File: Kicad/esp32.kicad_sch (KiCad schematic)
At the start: 25 parts, among them J2 Display, J3 LED, J7 UART, U11 ESP32-WROOM-32UE-N16, U16 XL1509-3.3

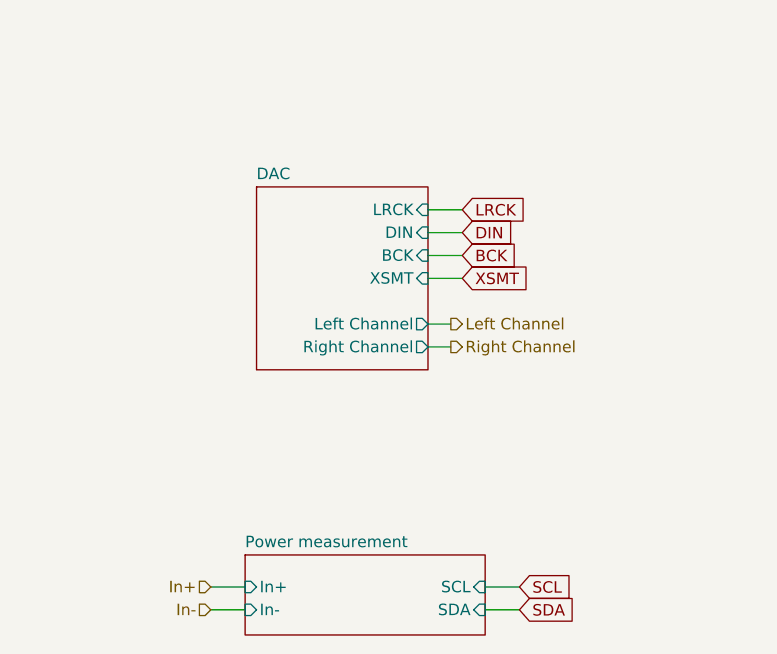
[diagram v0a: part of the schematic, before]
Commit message: final schematic
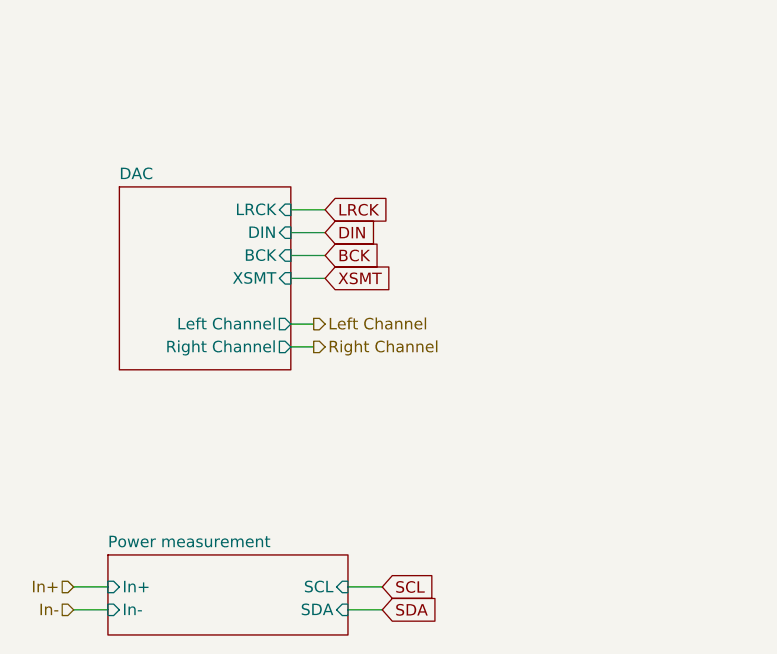
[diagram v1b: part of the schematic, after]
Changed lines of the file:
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@@
 	(wire
 		(pts
-			(xy 82.55 129.54) (xy 85.09 129.54)
+			(xy 67.31 129.54) (xy 69.85 129.54)
 		)
 		(stroke
@@
 	(wire
 		(pts
-			(xy 82.55 121.92) (xy 86.36 121.92)
+			(xy 67.31 121.92) (xy 71.12 121.92)
 		)
 		(stroke
@@
 	(wire
 		(pts
-			(xy 82.55 127) (xy 85.09 127)
+			(xy 67.31 127) (xy 69.85 127)
 		)
 		(stroke
@@
 	(wire
 		(pts
-			(xy 58.42 156.21) (xy 62.23 156.21)
+			(xy 43.18 156.21) (xy 46.99 156.21)
 		)
 		(stroke
@@
 	(wire
 		(pts
-			(xy 92.71 158.75) (xy 88.9 158.75)
+			(xy 77.47 158.75) (xy 73.66 158.75)
 		)
 		(stroke
@@
 	(wire
 		(pts
-			(xy 82.55 116.84) (xy 86.36 116.84)
+			(xy 67.31 116.84) (xy 71.12 116.84)
 		)
 		(stroke
@@
 	(wire
 		(pts
-			(xy 58.42 158.75) (xy 62.23 158.75)
+			(xy 43.18 158.75) (xy 46.99 158.75)
 		)
 		(stroke
@@
 	(wire
 		(pts
-			(xy 82.55 114.3) (xy 86.36 114.3)
+			(xy 67.31 114.3) (xy 71.12 114.3)
 		)
 		(stroke
@@
 	(wire
 		(pts
-			(xy 92.71 156.21) (xy 88.9 156.21)
+			(xy 77.47 156.21) (xy 73.66 156.21)
 		)
 		(stroke
@@
 	(wire
 		(pts
-			(xy 82.55 119.38) (xy 86.36 119.38)
+			(xy 67.31 119.38) (xy 71.12 119.38)
 		)
 		(stroke
@@
 	(global_label "BCK"
 		(shape input)
-		(at 86.36 119.38 0)
+		(at 71.12 119.38 0)
 		(fields_autoplaced yes)
 		(effects
@@
 		)
 		(property "Intersheetrefs" "${INTERSHEET_REFS}"
-			(at 93.1552 119.38 0)
+			(at 77.9152 119.38 0)
 			(hide yes)
 			(show_name no)
@@
 	(global_label "SCL"
 		(shape input)
-		(at 92.71 156.21 0)
+		(at 77.47 156.21 0)
 		(fields_autoplaced yes)
 		(effects
@@
 		)
 		(property "Intersheetrefs" "${INTERSHEET_REFS}"
-			(at 99.2028 156.21 0)
+			(at 83.9628 156.21 0)
 			(hide yes)
 			(show_name no)
@@
 	(global_label "XSMT"
 		(shape input)
-		(at 86.36 121.92 0)
+		(at 71.12 121.92 0)
 		(fields_autoplaced yes)
 		(effects
@@
 		)
 		(property "Intersheetrefs" "${INTERSHEET_REFS}"
-			(at 94.1832 121.92 0)
+			(at 78.9432 121.92 0)
 			(hide yes)
 			(show_name no)
@@
 	(global_label "SDA"
 		(shape input)
-		(at 92.71 158.75 0)
+		(at 77.47 158.75 0)
 		(fields_autoplaced yes)
 		(effects
@@
 		)
 		(property "Intersheetrefs" "${INTERSHEET_REFS}"
-			(at 99.2633 158.75 0)
+			(at 84.0233 158.75 0)
 			(hide yes)
 			(show_name no)
@@
 	(global_label "LRCK"
 		(shape input)
-		(at 86.36 114.3 0)
+		(at 71.12 114.3 0)
 		(fields_autoplaced yes)
 		(effects
@@
 		)
 		(property "Intersheetrefs" "${INTERSHEET_REFS}"
-			(at 94.1833 114.3 0)
+			(at 78.9433 114.3 0)
 			(hide yes)
 			(show_name no)
@@
 	(global_label "DIN"
 		(shape input)
-		(at 86.36 116.84 0)
+		(at 71.12 116.84 0)
 		(fields_autoplaced yes)
 		(effects
@@
 		)
 		(property "Intersheetrefs" "${INTERSHEET_REFS}"
-			(at 92.5505 116.84 0)
+			(at 77.3105 116.84 0)
 			(hide yes)
 			(show_name no)
@@
 	(hierarchical_label "Left Channel"
 		(shape output)
-		(at 85.09 127 0)
+		(at 69.85 127 0)
 		(effects
 			(font
@@
 	(hierarchical_label "Right Channel"
 		(shape output)
-		(at 85.09 129.54 0)
+		(at 69.85 129.54 0)
 		(effects
 			(font
@@
 	(hierarchical_label "In-"
 		(shape input)
-		(at 58.42 158.75 180)
+		(at 43.18 158.75 180)
 		(effects
 			(font
@@
 	(hierarchical_label "In+"
 		(shape input)
-		(at 58.42 156.21 180)
+		(at 43.18 156.21 180)
 		(effects
 			(font
@@
 	)
 	(sheet
-		(at 63.5 111.76)
+		(at 48.26 111.76)
 		(size 19.05 20.32)
 		(exclude_from_sim no)
@@
 		)
 		(property "Sheetname" "DAC"
-			(at 63.5 111.0484 0)
+			(at 48.26 111.0484 0)
 			(show_name no)
 			(do_not_autoplace no)
@@
 		)
 		(property "Sheetfile" "dac.kicad_sch"
-			(at 63.5 132.6646 0)
+			(at 48.26 132.6646 0)
 			(hide yes)
 			(show_name no)
@@
 		)
 		(pin "Right Channel" output
-			(at 82.55 129.54 0)
+			(at 67.31 129.54 0)
 			(effects
 				(font
@@
 		)
 		(pin "Left Channel" output
-			(at 82.55 127 0)
+			(at 67.31 127 0)
 			(effects
 				(font
@@
 		)
 		(pin "LRCK" input
-			(at 82.55 114.3 0)
+			(at 67.31 114.3 0)
 			(effects
 				(font
@@
 		)
 		(pin "BCK" input
-			(at 82.55 119.38 0)
+			(at 67.31 119.38 0)
 			(effects
 				(font
@@
 		)
 		(pin "DIN" input
-			(at 82.55 116.84 0)
+			(at 67.31 116.84 0)
 			(effects
 				(font
@@
 		)
 		(pin "XSMT" input
-			(at 82.55 121.92 0)
+			(at 67.31 121.92 0)
 			(effects
 				(font
@@
 	)
 	(sheet
-		(at 62.23 152.654)
+		(at 46.99 152.654)
 		(size 26.67 8.89)
 		(exclude_from_sim no)
@@
 		)
 		(property "Sheetname" "Power measurement"
-			(at 62.23 151.9424 0)
+			(at 46.99 151.9424 0)
 			(show_name no)
 			(do_not_autoplace no)
@@
 		)
 		(property "Sheetfile" "Power measurement.kicad_sch"
-			(at 62.23 162.1286 0)
+			(at 46.99 162.1286 0)
 			(hide yes)
 			(show_name no)
@@
 		)
 		(pin "SDA" input
-			(at 88.9 158.75 0)
+			(at 73.66 158.75 0)
 			(effects
 				(font
@@
 		)
 		(pin "SCL" input
-			(at 88.9 156.21 0)
+			(at 73.66 156.21 0)
 			(effects
 				(font
@@
 		)
 		(pin "In+" input
-			(at 62.23 156.21 180)
+			(at 46.99 156.21 180)
 			(effects
 				(font
@@
 		)
 		(pin "In-" input
-			(at 62.23 158.75 180)
+			(at 46.99 158.75 180)
 			(effects
 				(font
